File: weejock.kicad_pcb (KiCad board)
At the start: 2 copper layers, 44 parts, among them J2 JST-PH2, K1 PG1350, K10 PG1350, K11 PG1350, K12 PG1350, K13 PG1350, K14 PG1350, K15 PG1350, K16 PG1350, K17 PG1350, K18 PG1350, K19 PG1350, K2 PG1350, K20 PG1350, K3 PG1350, K4 PG1350, K5 PG1350, K6 PG1350, K7 PG1350, K8 PG1350, K9 PG1350, SW1 SW_Push, SW2 SW_SPDT, U1 Seeed Studio XIAO nRF52840

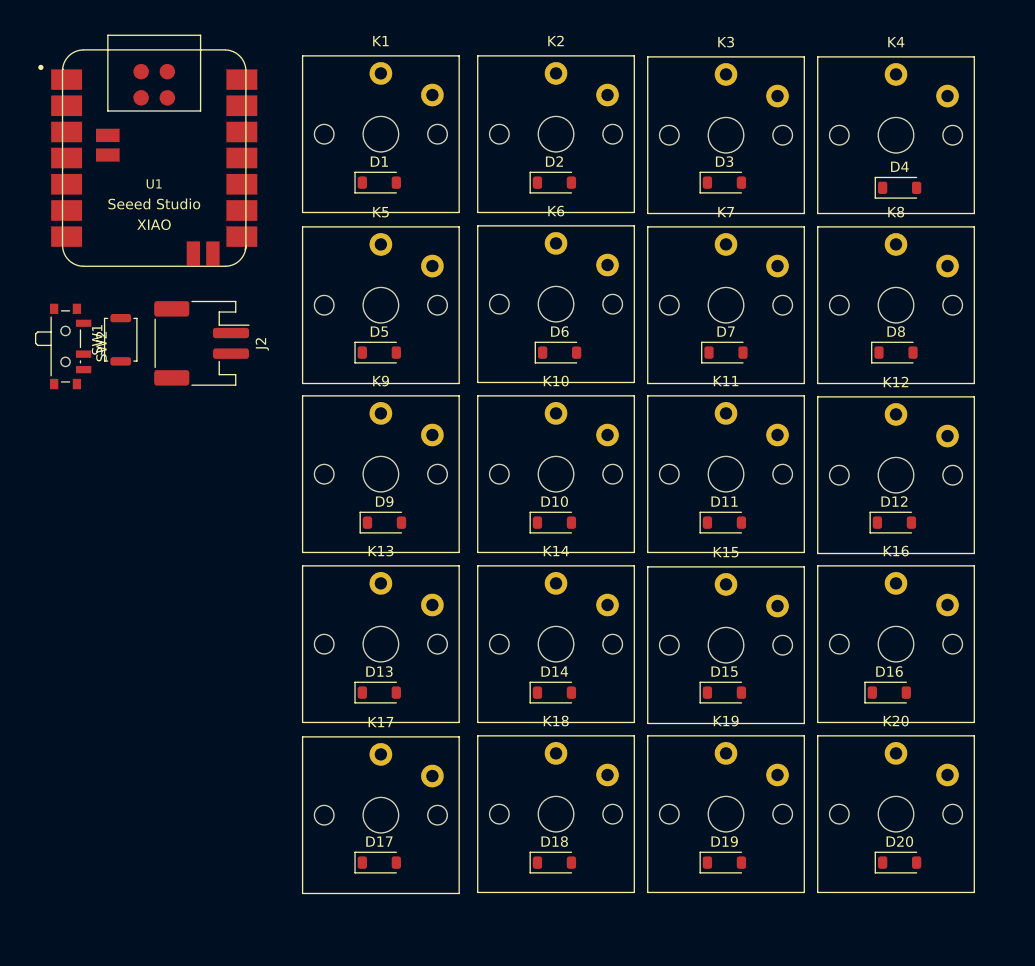
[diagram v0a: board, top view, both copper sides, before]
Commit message: Routing traces.
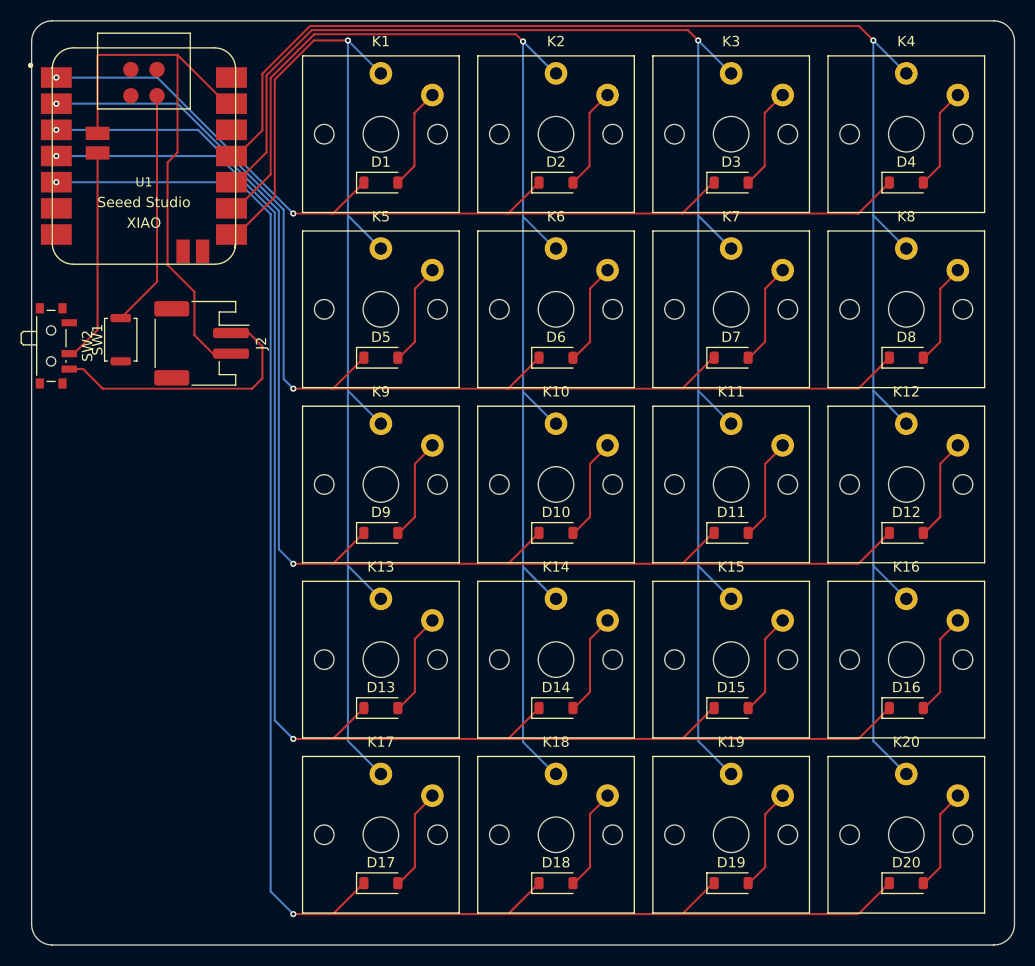
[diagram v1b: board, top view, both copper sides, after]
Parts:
- moved K20 2.24 mm to (159.5, 126.3)
- moved D16 2.23 mm to (159.5, 114.0)
- moved D19 2.10 mm to (142.5, 131.0)
- moved D20 2.10 mm to (159.5, 131.0)
- moved K19 2.06 mm to (142.5, 126.3)
- moved D17 2.01 mm to (108.5, 131.0)
- moved D18 2.01 mm to (125.5, 131.0)
- moved K18 2.00 mm to (125.5, 126.3)
- moved K17 1.90 mm to (108.5, 126.3)
- moved K16 1.80 mm to (159.5, 109.3)
- moved D15 1.63 mm to (142.5, 114.0)
- moved D12 1.52 mm to (159.5, 97.0)
- moved D13 1.51 mm to (108.5, 114.0)
- moved D14 1.51 mm to (125.5, 114.0)
- moved K13 1.50 mm to (108.5, 109.3)
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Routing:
- net row4: track 0.00 -> 162.7 mm, vias 0 -> 2
- net col3: track 0.00 -> 161.9 mm, vias 0 -> 1
- net row3: track 0.00 -> 147.0 mm, vias 0 -> 2
- net col2: track 0.00 -> 146.8 mm, vias 0 -> 1
- net col1: track 0.00 -> 131.7 mm, vias 0 -> 1
- net row2: track 0.00 -> 131.4 mm, vias 0 -> 2
- net col0: track 0.00 -> 117.0 mm, vias 0 -> 1
- net row1: track 0.00 -> 115.8 mm, vias 0 -> 2
- net row0: track 0.00 -> 100.5 mm, vias 0 -> 2
- net GND: track 0.00 -> 55.5 mm
- net Net-(J2-Pin_1): track 0.00 -> 26.6 mm
- net RST: track 0.00 -> 23.0 mm
- net BAT+: track 0.00 -> 20.9 mm
- net Net-(D20-A): track 0.00 -> 9.89 mm
- net Net-(D19-A): track 0.00 -> 9.89 mm
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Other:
- board outline added: 95.4 x 89.7 mm
